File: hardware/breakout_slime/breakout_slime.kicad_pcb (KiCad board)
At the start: 2 copper layers, 54.6 x 35.6 mm, 11 parts, among them J1 Battery_Connector, J2 IMU_Conn_Female, SW1 SW_SPDT, U1 TP4056_Breakout, U2 WeMos_D1_mini, U3 BNO/MPU_Break

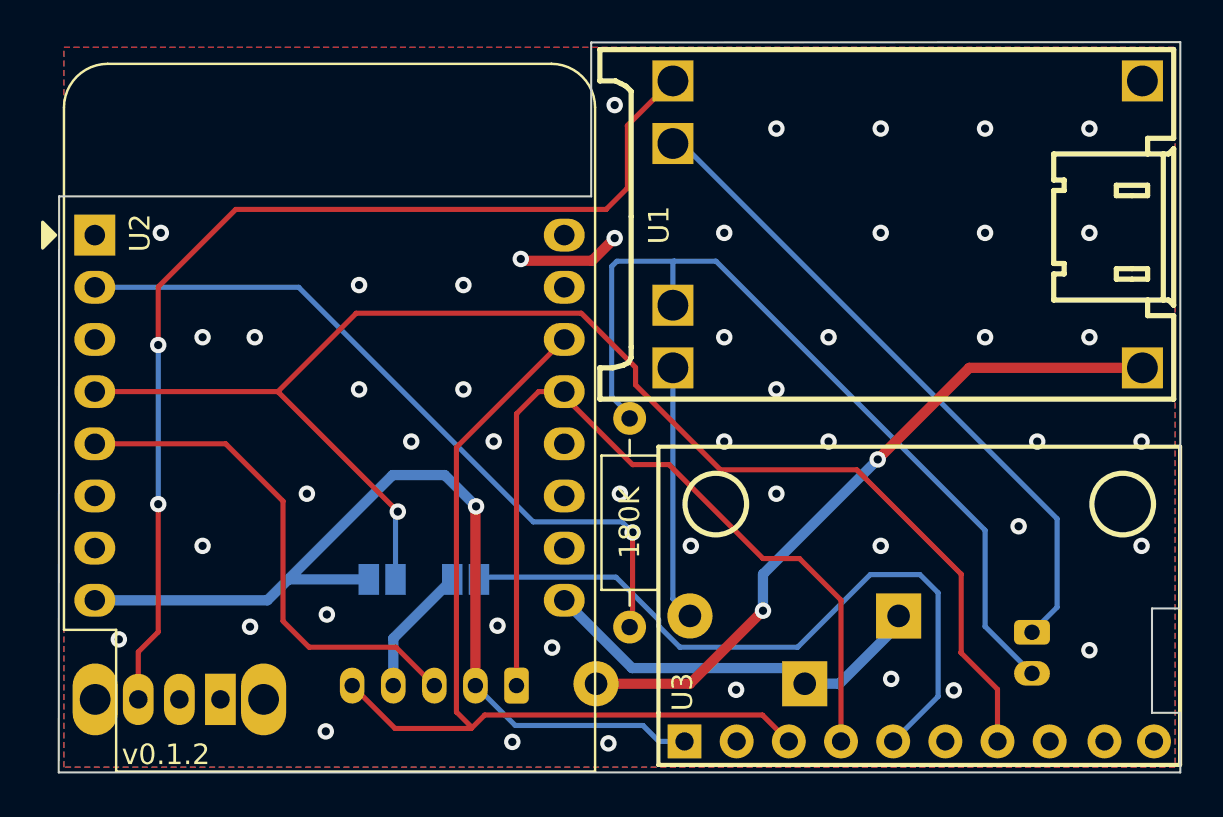
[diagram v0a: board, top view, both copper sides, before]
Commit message: [breakout_slime] Released v0.1.3
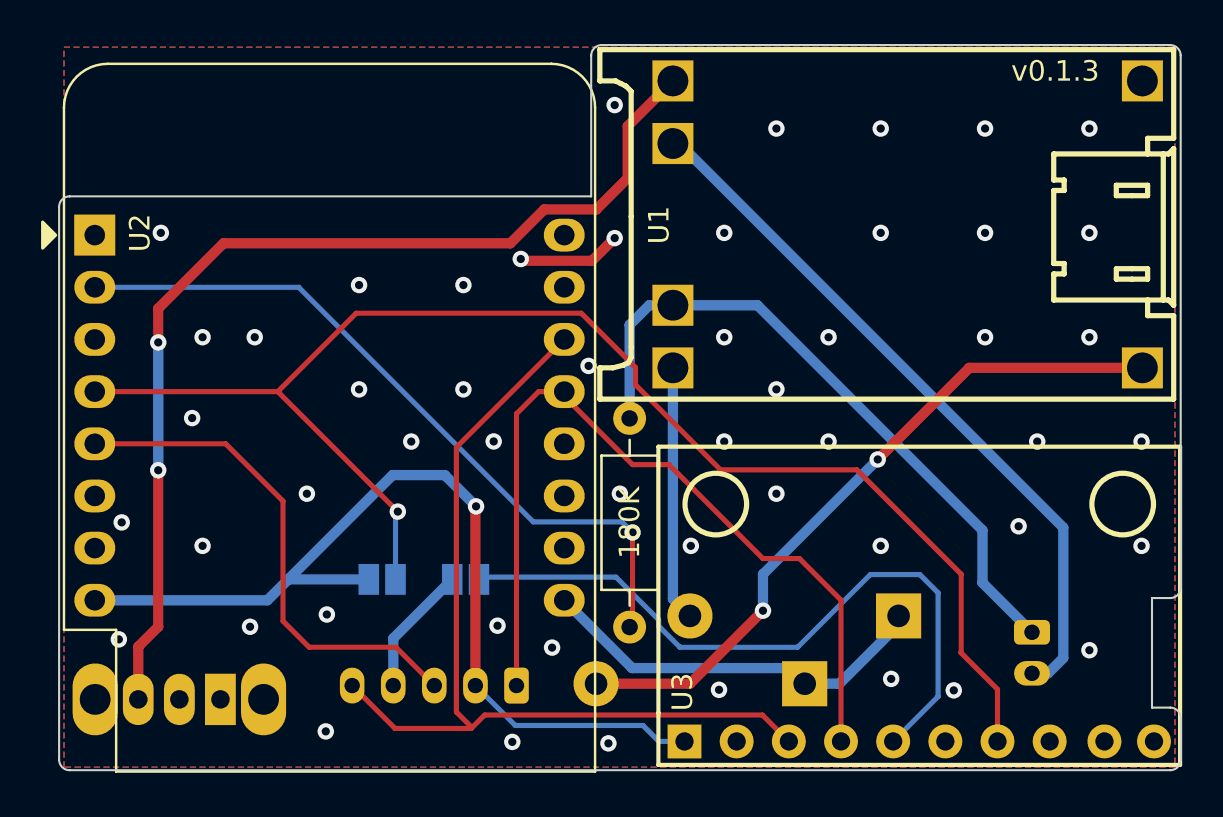
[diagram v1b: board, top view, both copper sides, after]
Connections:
- J1 pad 1: Net-(J1-Pad1) -> B+
- J1 pad 2: B+ -> Net-(J1-Pad2)
- U1 pad 4: Net-(J1-Pad1) -> Net-(J1-Pad2)
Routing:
- net Net-(J1-Pad2): track 0.00 -> 34.6 mm
- net Net-(J1-Pad1): track 31.9 -> 0.00 mm
- net B+: track 41.6 -> 32.6 mm
- net Net-(SW1-Pad3): track 51.4 -> 50.6 mm
- net GND: vias 49 -> 52
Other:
- board size 54.6 x 35.6 mm -> 54.6 x 35.3 mm
- board text added: "B+"
- board text added: "B-"
